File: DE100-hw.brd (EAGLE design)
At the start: 96.5 x 71.8 mm, 51 parts, among them IC3 74HC14D, IC4 74HC14D, U1 TLP521-4(GB), U2 TLP521-4(GB), X1 22-23-2041, X2 22-23-2031, X3 22-23-2101

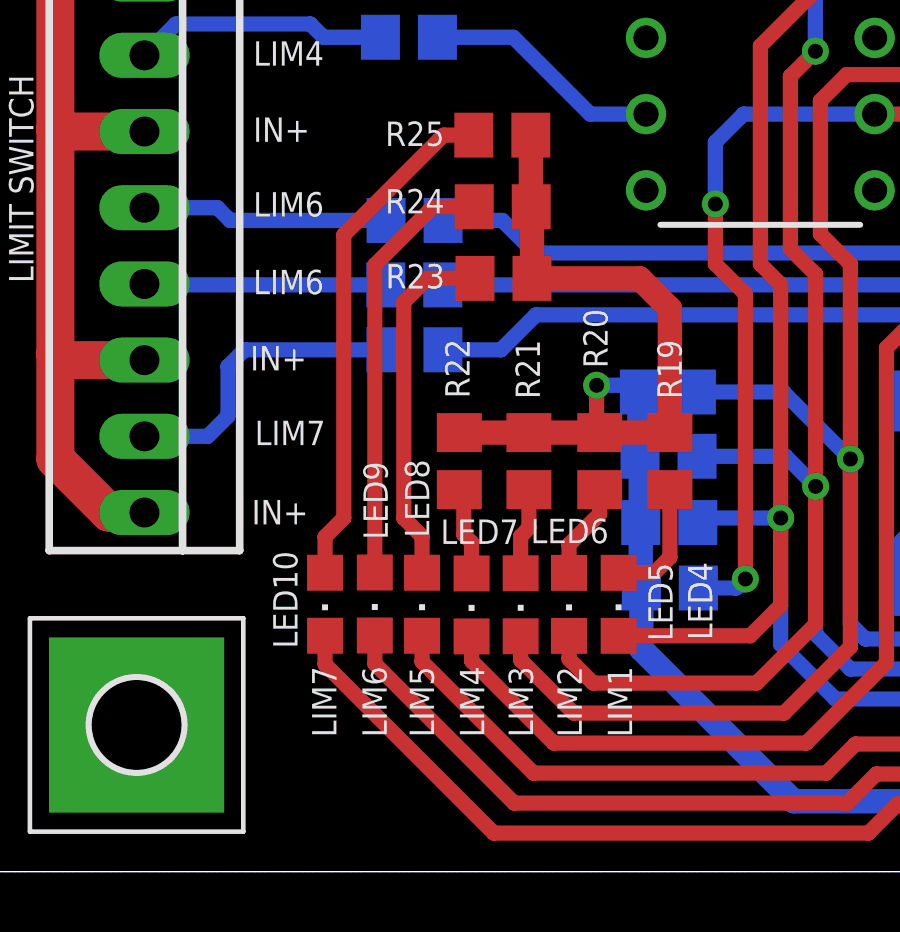
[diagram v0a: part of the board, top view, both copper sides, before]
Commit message: post production revision
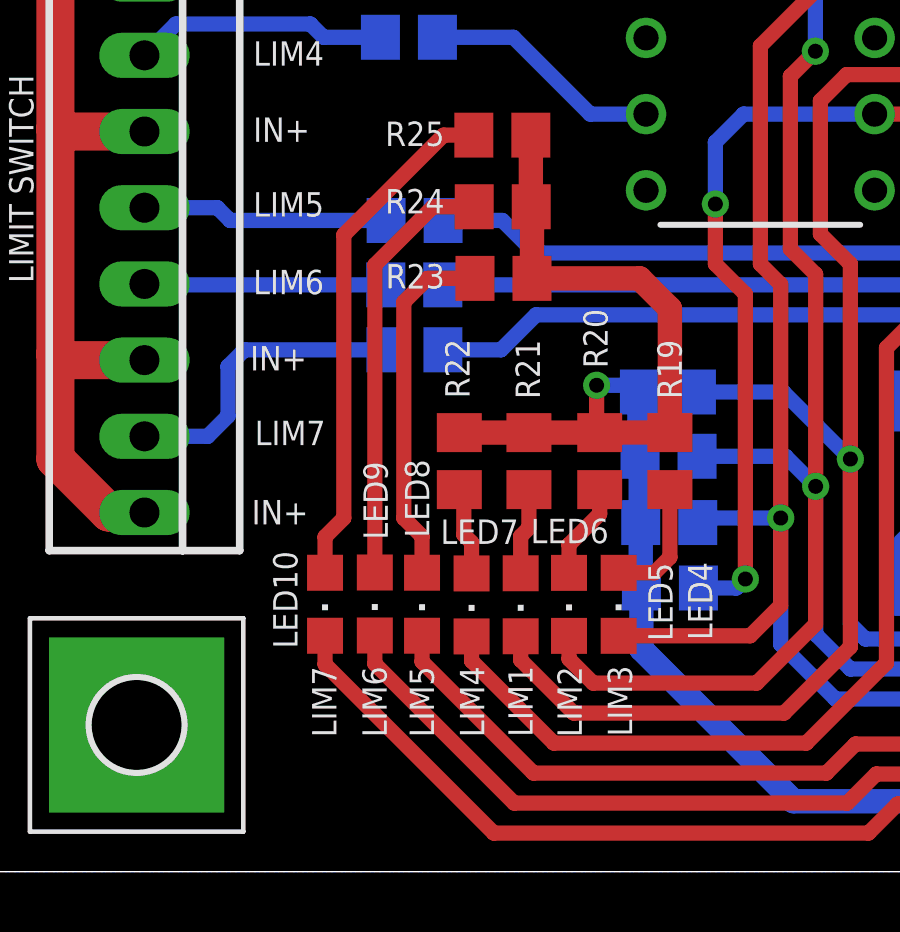
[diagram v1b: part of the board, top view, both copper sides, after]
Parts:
- R1, R10, R11, R18, R2, R26, R27, R3, R4, R9: value (none) -> 330
- R12, R13, R14, R5, R6, R7, R8: value (none) -> 10k
- R15, R16, R17, R19, R20, R21, R22, R23, R24, R25: value (none) -> 1k
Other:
- board text added: "Designed by:"
